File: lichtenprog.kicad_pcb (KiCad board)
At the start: 2 copper layers, 22 x 32 mm, 16 parts, among them J1 USB_B_Mini, J2 Conn_01x06, U1 AMS1117-3.3, U2 CP2102N-A01-GQFN28

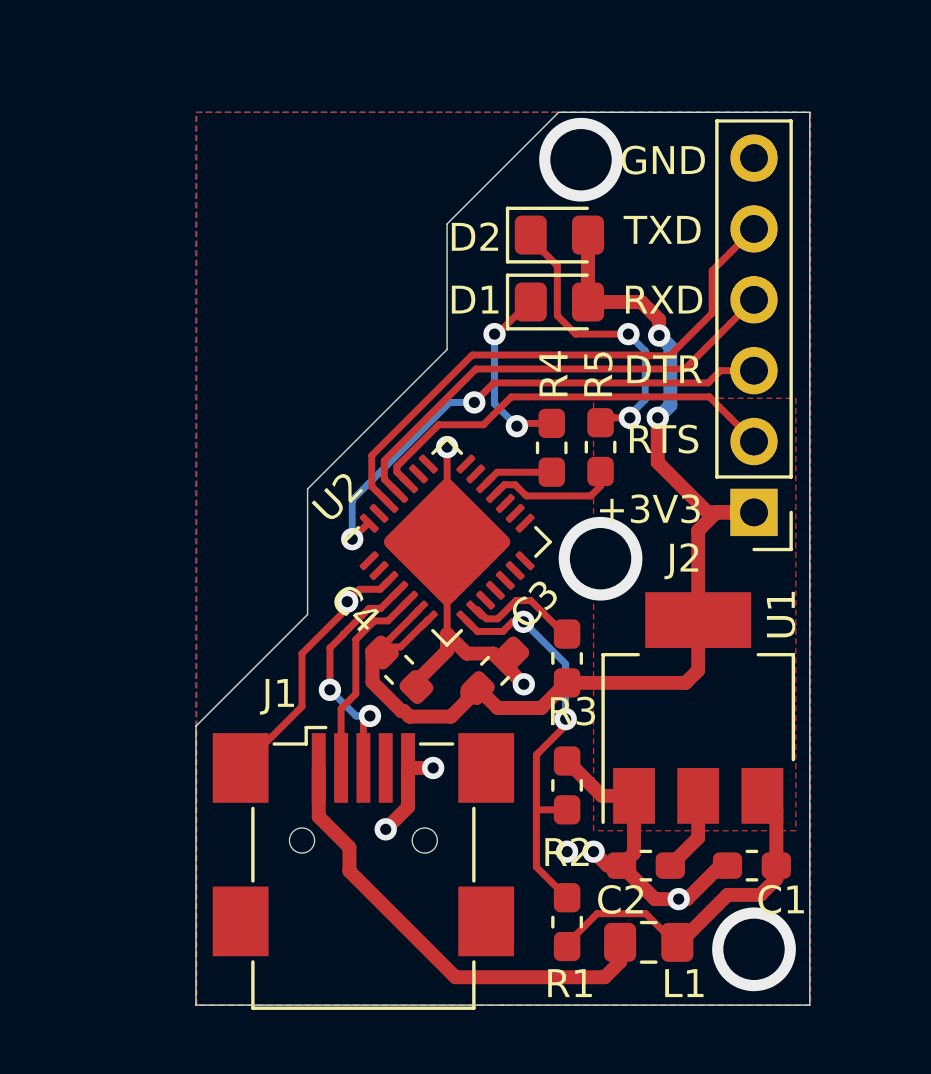
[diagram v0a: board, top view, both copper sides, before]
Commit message: rev 2 schematic and PCB do-over
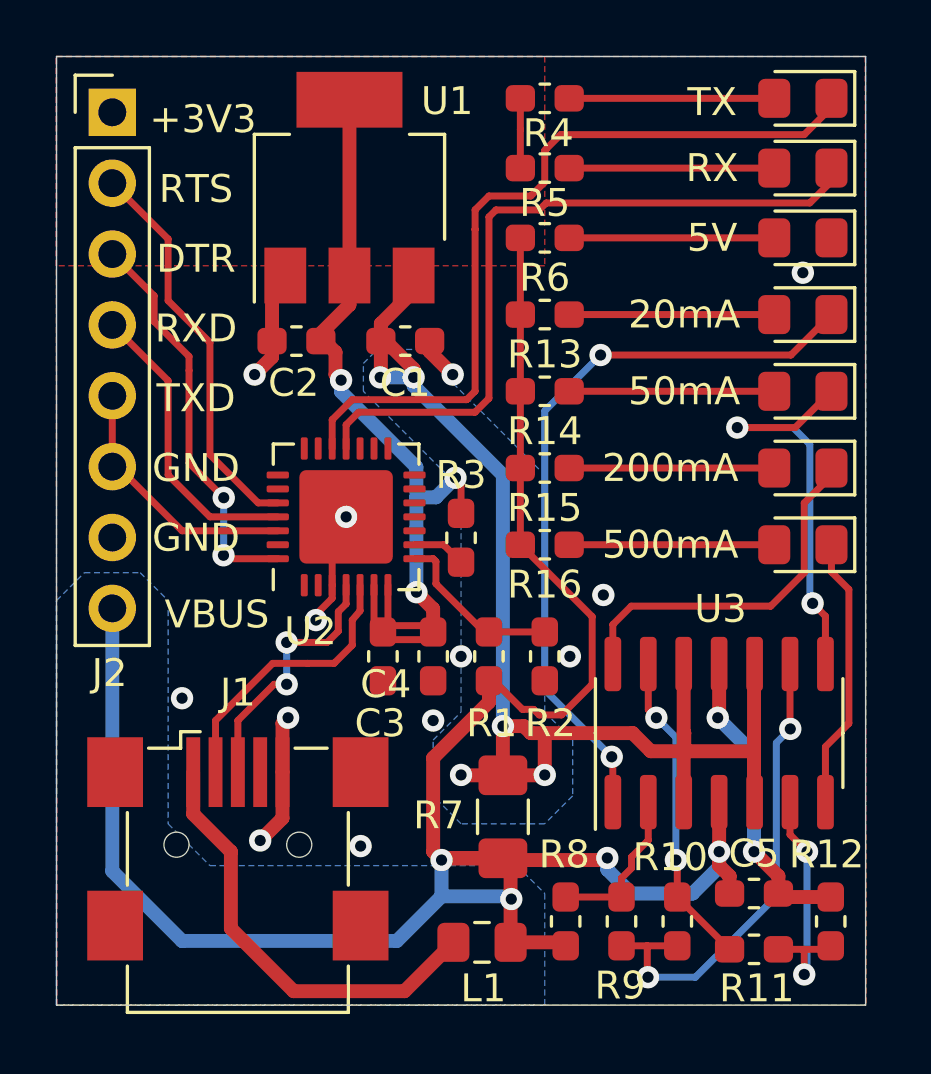
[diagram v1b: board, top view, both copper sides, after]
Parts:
- added C5: 100n, Capacitor_SMD:C_0603_1608Metric_Pad1.05x0.95mm_HandSolder, F.Cu at (89.0, 76.0)
- added D3: LED, LED_SMD:LED_0805_2012Metric_Pad1.15x1.40mm_HandSolder, F.Cu at (90.8, 52.5)
- added D4: LED, LED_SMD:LED_0805_2012Metric_Pad1.15x1.40mm_HandSolder, F.Cu at (90.8, 55.2)
- added D5: LED, LED_SMD:LED_0805_2012Metric_Pad1.15x1.40mm_HandSolder, F.Cu at (90.8, 58.0)
- added D6: LED, LED_SMD:LED_0805_2012Metric_Pad1.15x1.40mm_HandSolder, F.Cu at (90.8, 60.8)
- added D7: LED, LED_SMD:LED_0805_2012Metric_Pad1.15x1.40mm_HandSolder, F.Cu at (90.8, 63.5)
- added R10: 1.5k, Resistor_SMD:R_0603_1608Metric_Pad1.05x0.95mm_HandSolder, F.Cu at (86.2, 77.0)
- added R11: 3k, Resistor_SMD:R_0603_1608Metric_Pad1.05x0.95mm_HandSolder, F.Cu at (89.0, 78.0)
- added R12: 45k, Resistor_SMD:R_0603_1608Metric_Pad1.05x0.95mm_HandSolder, F.Cu at (91.8, 77.0)
- added R13: 1k, Resistor_SMD:R_0603_1608Metric_Pad1.05x0.95mm_HandSolder, F.Cu at (81.5, 55.2)
- added R14: 1k, Resistor_SMD:R_0603_1608Metric_Pad1.05x0.95mm_HandSolder, F.Cu at (81.5, 58.0)
- added R15: 1k, Resistor_SMD:R_0603_1608Metric_Pad1.05x0.95mm_HandSolder, F.Cu at (81.5, 60.8)
- added R16: 1k, Resistor_SMD:R_0603_1608Metric_Pad1.05x0.95mm_HandSolder, F.Cu at (81.5, 63.5)
- added R6: 1k, Resistor_SMD:R_0603_1608Metric_Pad1.05x0.95mm_HandSolder, F.Cu at (81.5, 52.5)
- added R7: 1R, Resistor_SMD:R_1206_3216Metric_Pad1.42x1.75mm_HandSolder, F.Cu at (80.0, 73.2)
- added R8: 100, Resistor_SMD:R_0603_1608Metric_Pad1.05x0.95mm_HandSolder, F.Cu at (82.2, 77.0)
- added R9: 400, Resistor_SMD:R_0603_1608Metric_Pad1.05x0.95mm_HandSolder, F.Cu at (84.2, 77.0)
- added U3: MCP6L04x-xSL, Package_SO:SOIC-14_3.9x8.7mm_P1.27mm, F.Cu at (87.8, 70.2)
- J2: value Conn_01x06 -> Conn_01x08; footprint Connector_PinHeader_2.54mm:PinHeader_1x06_P2.54mm_Vertical -> Connector_PinHeader_2.54mm:PinHeader_1x08_P2.54mm_Vertical
- R4, R5: value R_Small -> 400
- moved J2 27.1 mm to (66.0, 48.0), turned to 0 degrees
- moved C2 22.6 mm to (72.6, 56.2)
- moved C1 22.5 mm to (76.5, 56.2), turned to 0 degrees
- moved U1 22.5 mm to (74.5, 50.7)
- moved R4 12.5 mm to (81.5, 47.5), turned to 0 degrees
- moved D1 11.4 mm to (90.8, 47.5), turned to 180 degrees
- moved R5 10.2 mm to (81.5, 50.0), turned to 0 degrees
- moved R1 9.93 mm to (79.5, 67.5)
- moved D2 9.05 mm to (90.8, 50.0), turned to 180 degrees
- moved L1 5.97 mm to (79.2, 77.8)
- moved R3 5.76 mm to (78.5, 63.2), turned to 270 degrees
- moved R2 4.69 mm to (81.5, 67.5), turned to 270 degrees
- moved J1 4.50 mm to (70.5, 74.2)
- moved C3 4.05 mm to (75.7, 67.5), turned to 270 degrees
- moved U2 3.73 mm to (74.4, 62.5), turned to 90 degrees
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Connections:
- C1 pad 1: VBUS -> Net-(C1-Pad1)
- D1 pad 2: +3V3 -> Net-(D1-Pad2)
- D2 pad 2: +3V3 -> Net-(D2-Pad2)
- R4 pad 1: Net-(D1-Pad1) -> +3V3
- R4 pad 2: Net-(R4-Pad2) -> Net-(D1-Pad2)
- R5 pad 1: Net-(D2-Pad1) -> +3V3
- R5 pad 2: Net-(R5-Pad2) -> Net-(D2-Pad2)
- U1 pad 3: VBUS -> Net-(C1-Pad1)
- U2 pad 18: Net-(R5-Pad2) -> Net-(D2-Pad1)
- U2 pad 19: Net-(R4-Pad2) -> Net-(D1-Pad1)
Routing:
- net VBUS: track 12.1 -> 78.7 mm, vias 0 -> 4
- net Net-(C1-Pad1): track 0.00 -> 47.8 mm, vias 0 -> 5
- net Net-(D4-Pad1): track 0.00 -> 26.7 mm, vias 0 -> 2
- net Net-(D1-Pad1): track 6.70 -> 28.4 mm, vias 2 -> 0
- net Net-(R10-Pad1): track 0.00 -> 17.5 mm, vias 0 -> 2
- net Net-(D2-Pad1): track 11.3 -> 26.1 mm, vias 2 -> 0
- net Net-(D5-Pad1): track 0.00 -> 14.9 mm, vias 0 -> 2
- net Net-(D6-Pad1): track 0.00 -> 13.2 mm
- net Net-(R10-Pad2): track 0.00 -> 11.4 mm, vias 0 -> 2
- net GND: track 36.7 -> 25.6 mm, vias 10 -> 15
- net /PROG_TXD: track 20.0 -> 9.31 mm
- net Net-(D7-Pad1): track 0.00 -> 9.83 mm
- net +3V3: track 44.1 -> 34.4 mm
- net Net-(R11-Pad2): track 0.00 -> 9.30 mm, vias 0 -> 2
- net Net-(R1-Pad2): track 14.9 -> 6.23 mm, vias 2 -> 0
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- added copper zone on B.Cu, net Net-(C1-Pad1)
- added copper zone on B.Cu, net VBUS
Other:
- board size 22 x 32 mm -> 29 x 34 mm
- board text added: "200mA"
- board text added: "20mA"
- board text added: "500mA"
- board text added: "50mA"
- board text added: "5V"
- board text added: "Lichtenprog rev 2.0"
- board text added: "RX"
- board text added: "TX"
- board text added: "VBUS"
- board text added: "critbit@"
- board text removed: "<- He's hungry."
- board text removed: "Lichtenprog rev 1.0"
- board text removed: "critbit"
